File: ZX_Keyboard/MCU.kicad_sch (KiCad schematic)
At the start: 21 parts, among them J1 DBG_UART, J2 DEBUG, SW1 RESET, U1 STM32F105R8Tx, Y1 8MHz

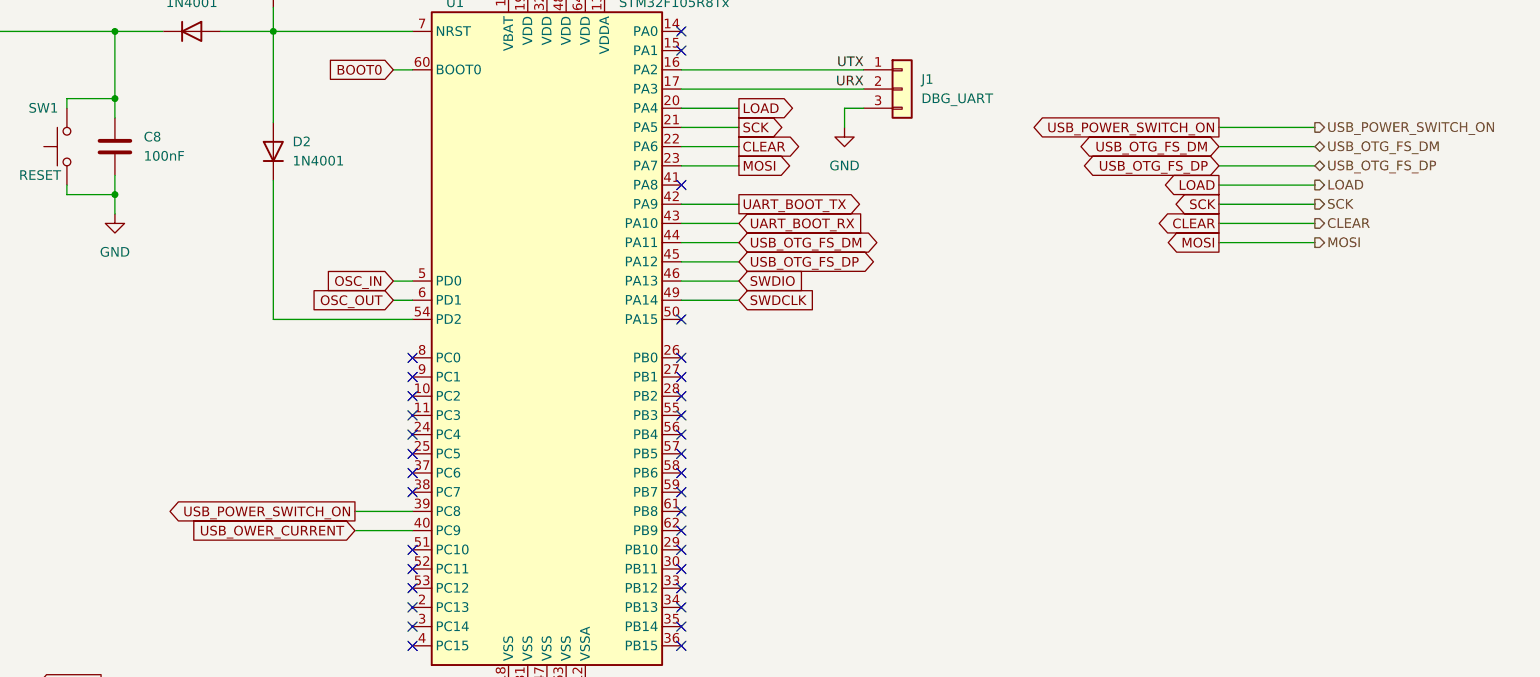
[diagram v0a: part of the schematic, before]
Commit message: update schematic and pcb
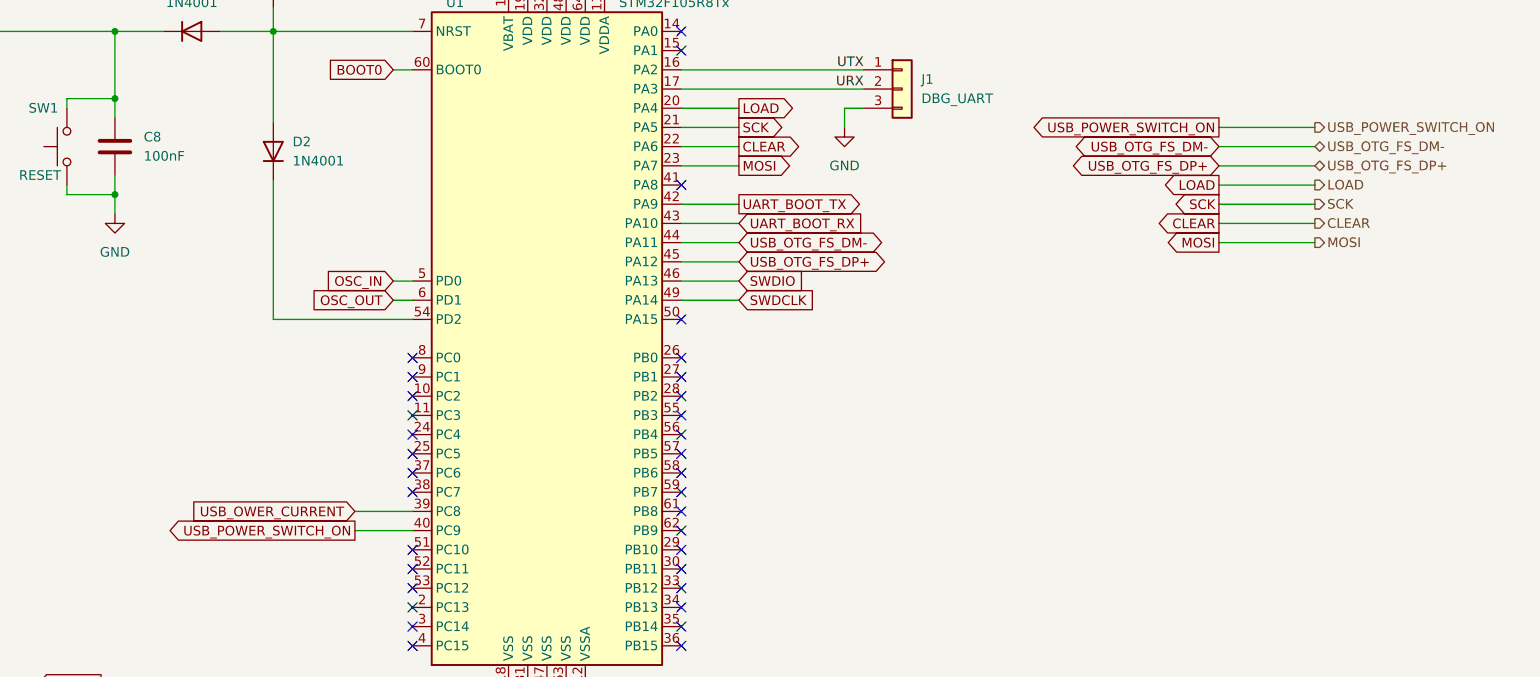
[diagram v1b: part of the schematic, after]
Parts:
- C7: footprint Capacitor_Tantalum_SMD:CP_EIA-3528-21_Kemet-B_Pad1.50x2.35mm_HandSolder -> Capacitor_Tantalum_SMD:CP_EIA-3216-18_Kemet-A_Pad1.58x1.35mm_HandSolder
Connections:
- net USB_OWER_CURRENT: now also U1.39 (PC8); no longer U1.40 (PC9)
- net USB_POWER_SWITCH_ON: now also U1.40 (PC9); no longer U1.39 (PC8)
- net USB_OTG_FS_DM renamed USB_OTG_FS_DM-
- net USB_OTG_FS_DP renamed USB_OTG_FS_DP+

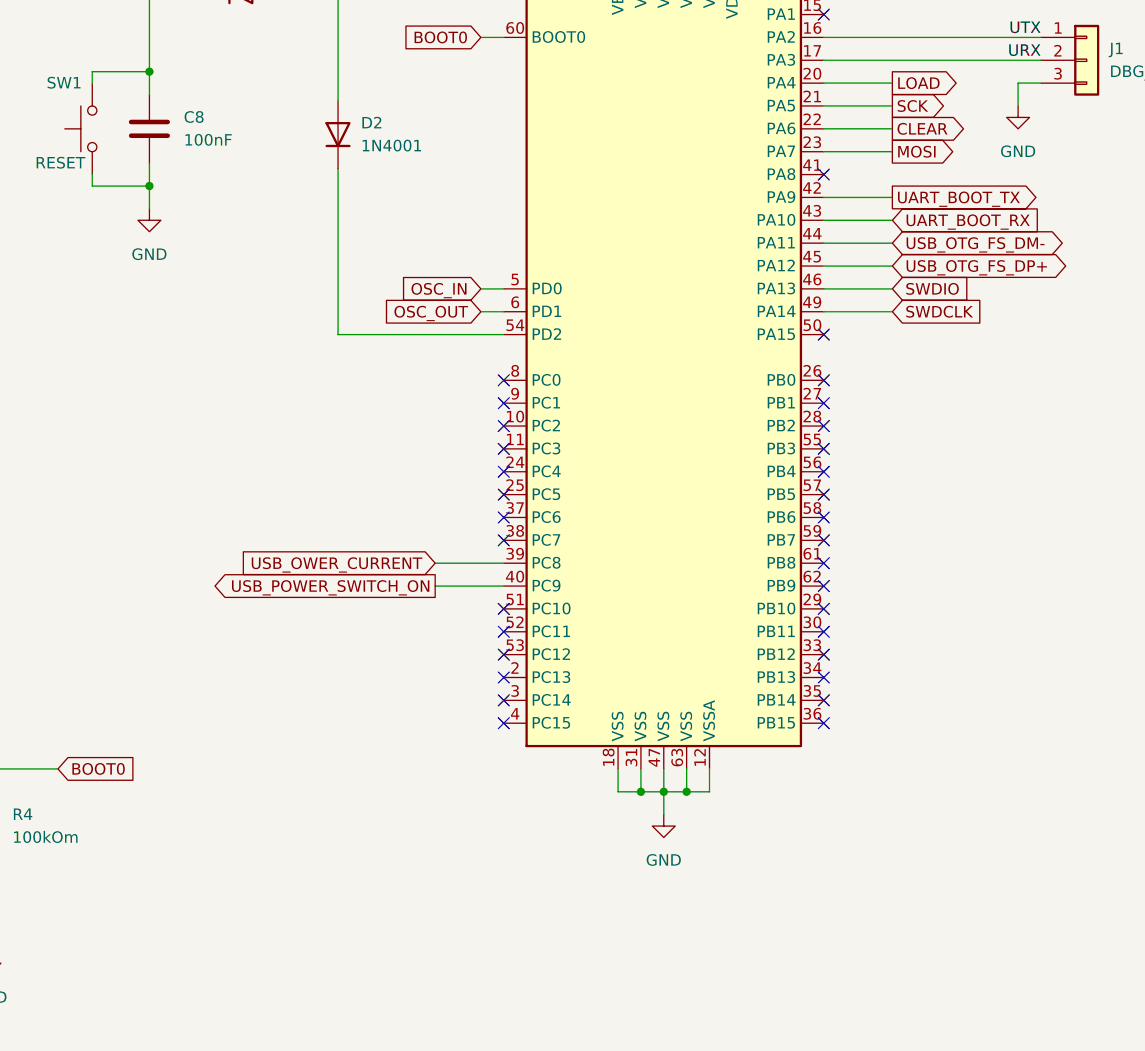
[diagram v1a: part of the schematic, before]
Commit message: update pcb
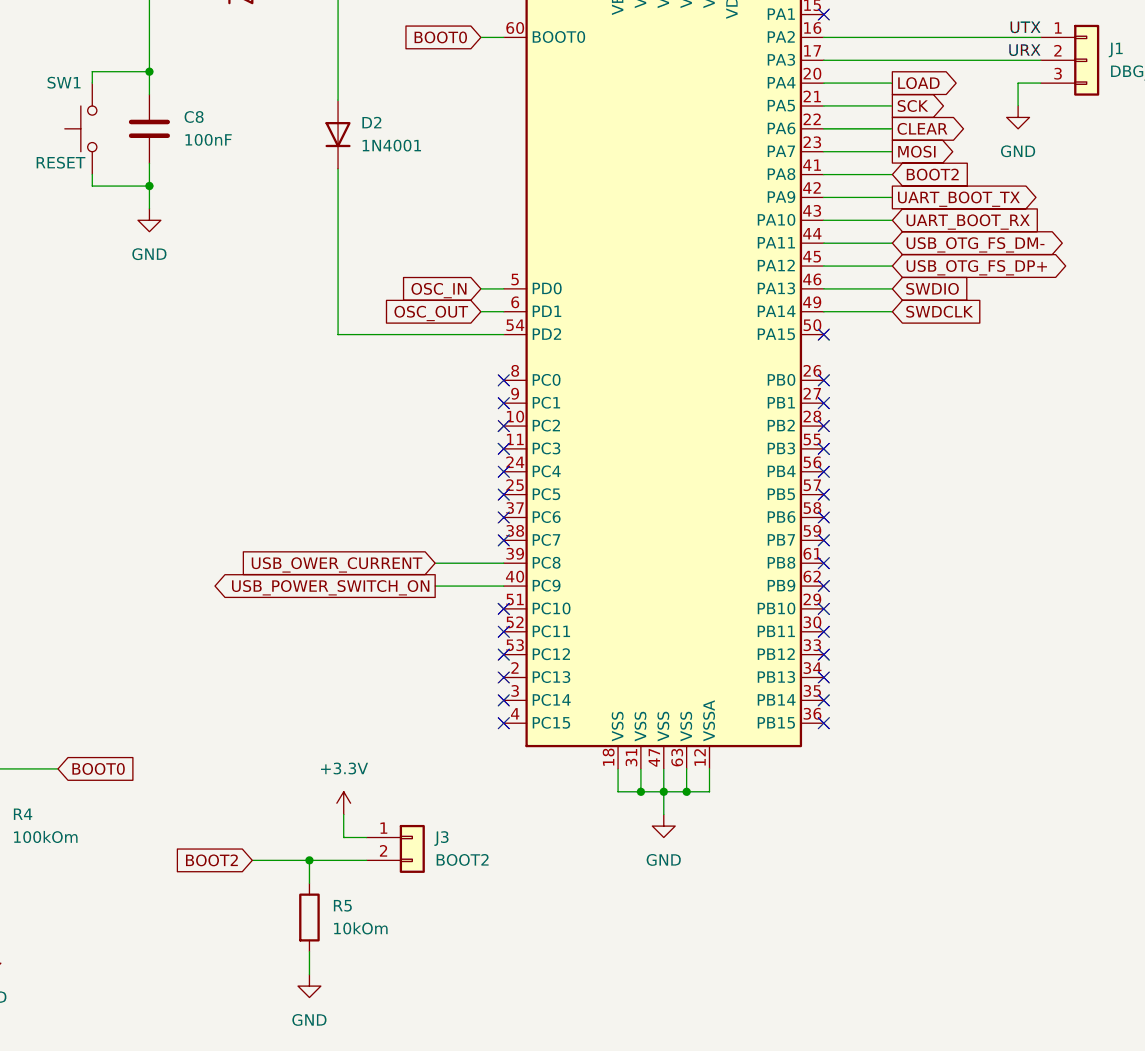
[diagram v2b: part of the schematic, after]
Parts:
- added J3: BOOT2, Connector_PinHeader_2.54mm:PinHeader_1x02_P2.54mm_Vertical, symbol Connector_Generic:Conn_01x02
- added R5: 10kOm, Resistor_SMD:R_0805_2012Metric_Pad1.20x1.40mm_HandSolder, symbol Device:R
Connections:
- net +3.3V: now also J3.1 (Pin_1)
- net GND: now also R5.2
- net BOOT2: now reaches U1.41 (PA8)
- net BOOT2: now also J3.2 (Pin_2), R5.1
- no-connect marks 34 -> 33
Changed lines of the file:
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@@
   (junction (at 154.94 68.58) (diameter 0) (color 0 0 0 0)
+  )
+  (junction (at 113.03 172.72) (diameter 0) (color 0 0 0 0)
   )
   (junction (at 154.94 165.1) (diameter 0) (color 0 0 0 0)
@@
   (no_connect (at 134.62 144.78))
   (no_connect (at 170.18 127))
-  (no_connect (at 170.18 96.52))
   (no_connect (at 170.18 142.24))
   (no_connect (at 134.62 119.38))
@@
     (stroke (width 0) (type default) (color 0 0 0 0))
   )
+  (wire (pts (xy 113.03 172.72) (xy 119.38 172.72))
+    (stroke (width 0) (type default) (color 0 0 0 0))
+  )
   (wire (pts (xy 50.8 127) (xy 50.8 129.54))
     (stroke (width 0) (type default) (color 0 0 0 0))
@@
     (stroke (width 0) (type default) (color 0 0 0 0))
   )
+  (wire (pts (xy 116.84 167.64) (xy 116.84 170.18))
+    (stroke (width 0) (type default) (color 0 0 0 0))
+  )
   (wire (pts (xy 50.8 137.16) (xy 50.8 139.7))
     (stroke (width 0) (type default) (color 0 0 0 0))
@@
     (stroke (width 0) (type default) (color 0 0 0 0))
   )
+  (wire (pts (xy 116.84 170.18) (xy 119.38 170.18))
+    (stroke (width 0) (type default) (color 0 0 0 0))
+  )
   (wire (pts (xy 241.3 93.98) (xy 254 93.98))
     (stroke (width 0) (type default) (color 0 0 0 0))
   )
+  (wire (pts (xy 113.03 172.72) (xy 113.03 175.26))
+    (stroke (width 0) (type default) (color 0 0 0 0))
+  )
   (wire (pts (xy 152.4 165.1) (xy 154.94 165.1))
     (stroke (width 0) (type default) (color 0 0 0 0))
@@
     (stroke (width 0) (type default) (color 0 0 0 0))
   )
+  (wire (pts (xy 106.68 172.72) (xy 113.03 172.72))
+    (stroke (width 0) (type default) (color 0 0 0 0))
+  )
   (wire (pts (xy 147.32 165.1) (xy 149.86 165.1))
     (stroke (width 0) (type default) (color 0 0 0 0))
@@
     (stroke (width 0) (type default) (color 0 0 0 0))
   )
+  (wire (pts (xy 113.03 182.88) (xy 113.03 185.42))
+    (stroke (width 0) (type default) (color 0 0 0 0))
+  )
   (wire (pts (xy 190.5 35.56) (xy 190.5 38.1))
     (stroke (width 0) (type default) (color 0 0 0 0))
@@
   )
   (wire (pts (xy 170.18 93.98) (xy 177.8 93.98))
+    (stroke (width 0) (type default) (color 0 0 0 0))
+  )
+  (wire (pts (xy 170.18 96.52) (xy 177.8 96.52))
     (stroke (width 0) (type default) (color 0 0 0 0))
   )
@@
     )
   )
+  (global_label "BOOT2" (shape input) (at 177.8 96.52 0) (fields_autoplaced)
+    (effects (font (size 1.27 1.27)) (justify left))
+    (property "Intersheet References" "${INTERSHEET_REFS}" (id 0) (at 186.3212 96.4406 0)
+      (effects (font (size 1.27 1.27)) (justify left) hide)
+    )
+  )
   (global_label "OSC_IN" (shape input) (at 63.5 114.3 0) (fields_autoplaced)
     (effects (font (size 1.27 1.27)) (justify left))
@@
     (effects (font (size 1.27 1.27)) (justify right))
     (property "Intersheet References" "${INTERSHEET_REFS}" (id 0) (at 216.2083 88.8206 0)
+      (effects (font (size 1.27 1.27)) (justify right) hide)
+    )
+  )
+  (global_label "BOOT2" (shape input) (at 106.68 172.72 180) (fields_autoplaced)
+    (effects (font (size 1.27 1.27)) (justify right))
+    (property "Intersheet References" "${INTERSHEET_REFS}" (id 0) (at 98.1588 172.6406 0)
       (effects (font (size 1.27 1.27)) (justify right) hide)
     )
@@
     (pin "2")
   )
+  (symbol (lib_id "Connector_Generic:Conn_01x02") (at 124.46 170.18 0) (unit 1)
+    (in_bom yes) (on_board yes) (fields_autoplaced)
+    (property "Reference" "J3" (id 0) (at 127 170.1799 0)
+      (effects (font (size 1.27 1.27)) (justify left))
+    )
+    (property "Value" "BOOT2" (id 1) (at 127 172.7199 0)
+      (effects (font (size 1.27 1.27)) (justify left))
+    )
+    (property "Footprint" "Connector_PinHeader_2.54mm:PinHeader_1x02_P2.54mm_Vertical" (id 2) (at 124.46 170.18 0)
+      (effects (font (size 1.27 1.27)) hide)
+    )
+    (property "Datasheet" "~" (id 3) (at 124.46 170.18 0)
+      (effects (font (size 1.27 1.27)) hide)
+    )
+    (pin "1")
+    (pin "2")
+  )
   (symbol (lib_id "Device:R") (at 57.15 114.3 90) (unit 1)
     (in_bom yes) (on_board yes)
@@
     (pin "1")
   )
+  (symbol (lib_id "power:GND") (at 113.03 185.42 0) (unit 1)
+    (in_bom yes) (on_board yes) (fields_autoplaced)
+    (property "Reference" "#PWR0101" (id 0) (at 113.03 191.77 0)
+      (effects (font (size 1.27 1.27)) hide)
+    )
+    (property "Value" "GND" (id 1) (at 113.03 190.5 0))
+    (property "Footprint" "" (id 2) (at 113.03 185.42 0)
+      (effects (font (size 1.27 1.27)) hide)
+    )
+    (property "Datasheet" "" (id 3) (at 113.03 185.42 0)
+      (effects (font (size 1.27 1.27)) hide)
+    )
+    (pin "1")
+  )
   (symbol (lib_id "power:+3.3V") (at 139.7 25.4 0) (unit 1)
     (in_bom yes) (on_board yes) (fields_autoplaced)
@@
     (pin "2")
   )
+  (symbol (lib_id "Device:R") (at 113.03 179.07 0) (unit 1)
+    (in_bom yes) (on_board yes) (fields_autoplaced)
+    (property "Reference" "R5" (id 0) (at 115.57 177.7999 0)
+      (effects (font (size 1.27 1.27)) (justify left))
+    )
+    (property "Value" "10kOm" (id 1) (at 115.57 180.3399 0)
+      (effects (font (size 1.27 1.27)) (justify left))
+    )
+    (property "Footprint" "Resistor_SMD:R_0805_2012Metric_Pad1.20x1.40mm_HandSolder" (id 2) (at 111.252 179.07 90)
+      (effects (font (size 1.27 1.27)) hide)
+    )
+    (property "Datasheet" "~" (id 3) (at 113.03 179.07 0)
+      (effects (font (size 1.27 1.27)) hide)
+    )
+    (pin "1")
+    (pin "2")
+  )
+  (symbol (lib_id "power:+3.3V") (at 116.84 167.64 0) (unit 1)
+    (in_bom yes) (on_board yes) (fields_autoplaced)
+    (property "Reference" "#PWR027" (id 0) (at 116.84 171.45 0)
+      (effects (font (size 1.27 1.27)) hide)
+    )
+    (property "Value" "+3.3V" (id 1) (at 116.84 162.56 0))
+    (property "Footprint" "" (id 2) (at 116.84 167.64 0)
+      (effects (font (size 1.27 1.27)) hide)
+    )
+    (property "Datasheet" "" (id 3) (at 116.84 167.64 0)
+      (effects (font (size 1.27 1.27)) hide)
+    )
+    (pin "1")
+  )
   (symbol (lib_id "power:GND") (at 127 38.1 0) (unit 1)
